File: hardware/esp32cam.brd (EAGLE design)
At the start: 33.5 x 34.6 mm, 45 parts, among them J1 MICRO_USB_B_HIROSE_ZX62-B-5PA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, Q1 HN1C01FU, U1 NJM11100, U2 NJM11100, U3 FT234XD-R, U4 NJM12888F, U6 SPU0414HR5H-SB

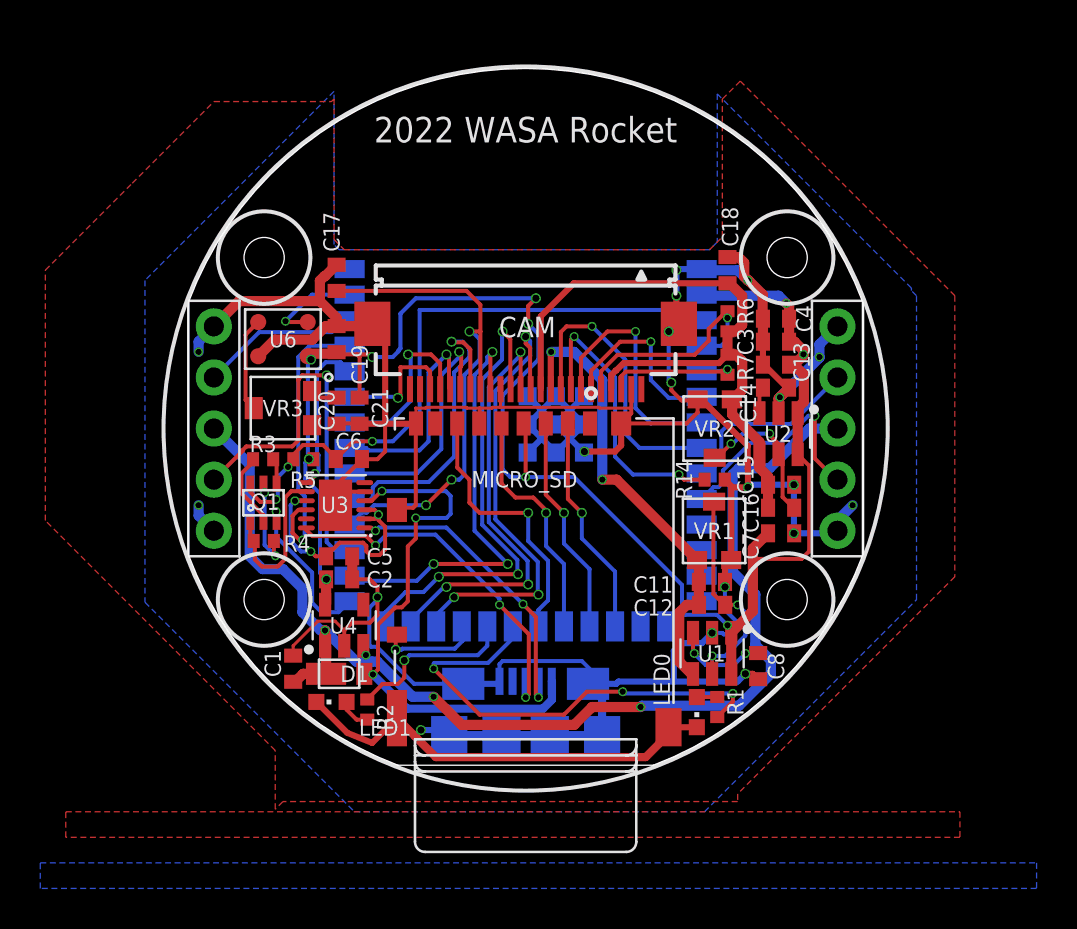
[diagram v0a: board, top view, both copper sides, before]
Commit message: 回路微修正
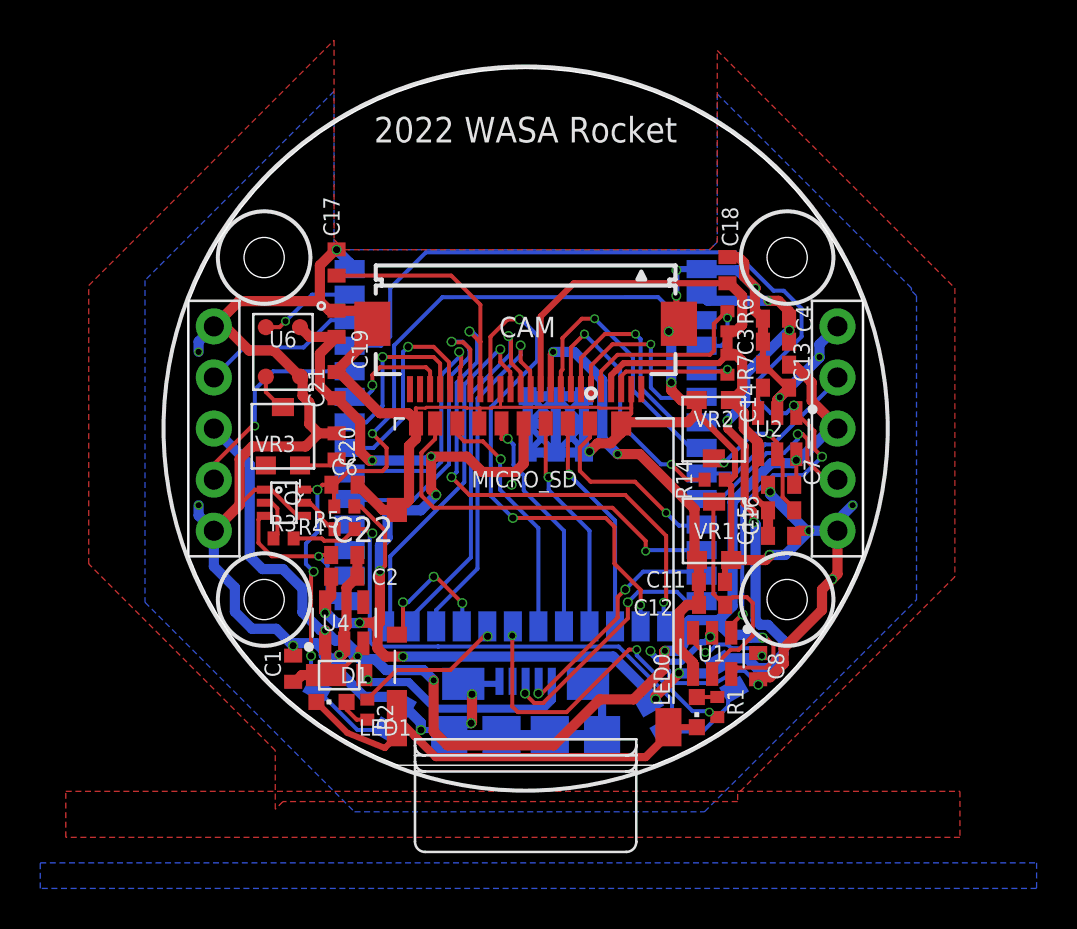
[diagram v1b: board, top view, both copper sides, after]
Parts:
- removed C5: 0.1µF, rcl:C0402
- removed U3: FT234XD-R, FT234XD-R:SON45P300X300X80-13N
- added C22: 1µF, rcl:C0402
- added PROG, RESET: THAF01-NC-R, switches:THAF01-NC-R
- R1, R2: value (none) -> 1k
- VR1, VR2: value (none) -> 100k
- moved R3 4.07 mm to (-12.0, -5.46)
- moved R4 4.06 mm to (-9.00, -5.00), turned to 180 degrees
- moved R5 3.11 mm to (-9.01, -3.88)
- moved C15 2.54 mm to (12.7, -5.33)
- moved C7 2.41 mm to (12.7, -2.79), turned to 180 degrees
- moved C20 1.78 mm to (-9.40, -0.89), turned to 90 degrees
- moved C21 1.71 mm to (-9.40, 2.16), turned to 90 degrees
- moved VR3 1.40 mm to (-12.1, -0.38), turned to 0 degrees
- moved C6 1.30 mm to (-9.00, -2.79)
- moved Q1 1.02 mm to (-12.0, -3.69), turned to 270 degrees
- moved C17 0.76 mm to (-9.40, 8.26)
- moved C19 0.76 mm to (-9.40, 5.21)
- moved U6 0.64 mm to (-12.1, 3.81), turned to 0 degrees
- moved C2 0.28 mm to (-9.02, -7.37)
- moved C16 0.13 mm to (12.7, -4.07)
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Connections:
- net 1.3V renamed 1.5V
- removed net DTR: Q1.4, R3.1
- removed net N$6: C5.1, U3.2, U3.3, U3.9
- removed net RTS: Q1.1, R4.1, U3.8
- removed net RTX: ESP32.36, U3.7
- removed net TRX: ESP32.37, U3.10
- new net CAM_POWER: ESP32.37, U1.1, U2.1
- new net N$5: PROG.3, PROG.4, R3.1, R4.1
- new net SDIO_D1: ESP32.12, MICRO_SD.8
- new net SDIO_D2: ESP32.11, MICRO_SD.1
- net D5: now also ESP32.16; no longer ESP32.28
- net EN: now also RESET.3, RESET.4
- net GND: now also C22.2, Q1.1, Q1.4, RESET.1, RESET.2; no longer C5.2, U3.13, U3.5
- net IO0: now also C22.1
- net PCLK: now also ESP32.15; no longer ESP32.30
- net RX0: now also ESP32.36; no longer ESP32.29
- net USB_DM: now also ESP32.13; no longer U3.1
- net USB_DP: now also ESP32.14; no longer U3.12
- net USB_VCC: no longer U3.4
- net V+: now also C13.1, C7.1, U1.6, U2.6
- net VDD: now also PROG.1, PROG.2; no longer C13.1, C7.1, U1.1, U1.6, U2.1, U2.6
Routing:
- net CAM_POWER: track 0.00 -> 49.3 mm, vias 0 -> 3
- net GND: track 201.8 -> 247.5 mm, vias 19 -> 25
- net N$5: track 0.00 -> 32.3 mm, vias 0 -> 1
- net SDIO_D1: track 0.00 -> 19.3 mm, vias 0 -> 1
- net USB_VCC: track 27.3 -> 11.2 mm, vias 3 -> 1
- net TRX: track 14.4 -> 0.00 mm, vias 1 -> 0
- net V+: track 60.1 -> 73.3 mm, vias 4 -> 6
- net EN: track 31.7 -> 44.6 mm, vias 3 -> 4
- net N$6: track 11.9 -> 0.00 mm, vias 3 -> 0
- net PCLK: track 26.6 -> 37.2 mm
- net SDIO_D2: track 0.00 -> 9.77 mm, vias 0 -> 1
- net RX0: track 19.2 -> 10.5 mm
- net RTX: track 8.10 -> 0.00 mm, vias 1 -> 0
- net RTS: track 8.02 -> 0.00 mm
- net D6: track 24.3 -> 18.4 mm, vias 3 -> 1
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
